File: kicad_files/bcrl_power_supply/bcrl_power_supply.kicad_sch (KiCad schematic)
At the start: 0 parts

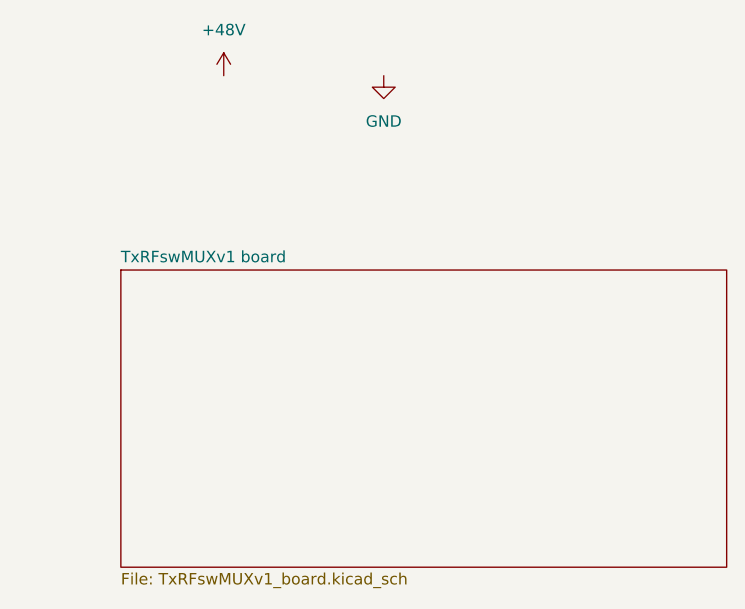
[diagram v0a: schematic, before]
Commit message: added decoupling
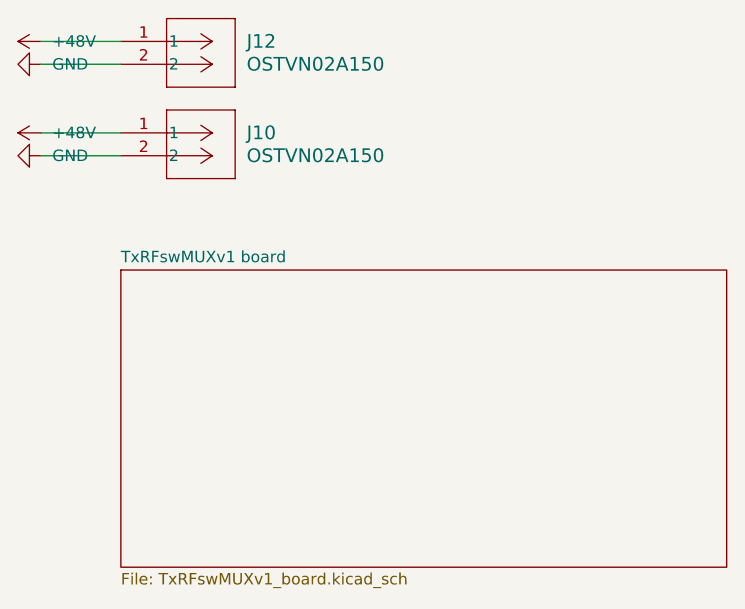
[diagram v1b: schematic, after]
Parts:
- added J10, J12: OSTVN02A150, symbol BCRL_power_supply:OSTVN02A150
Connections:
- net +48V: now also J10.1, J12.1
- net GND: now also J10.2, J12.2
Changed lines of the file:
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@@
 (kicad_sch (version 20230121) (generator eeschema)
   (paper "A4")
-  (symbol (lib_id "power:+48V") (at 50.8 27.94 0) (unit 1)
+  (wire (pts (xy 30.48 34.29) (xy 39.37 34.29))
+    (stroke (width 0) (type default))
+  )
+  (wire (pts (xy 30.48 24.13) (xy 39.37 24.13))
+    (stroke (width 0) (type default))
+  )
+  (wire (pts (xy 30.48 36.83) (xy 39.37 36.83))
+    (stroke (width 0) (type default))
+  )
+  (wire (pts (xy 30.48 26.67) (xy 39.37 26.67))
+    (stroke (width 0) (type default))
+  )
+  (symbol (lib_id "BCRL_power_supply:OSTVN02A150") (at 39.37 34.29 0) (unit 1)
     (in_bom yes) (on_board yes) (dnp no) (fields_autoplaced)
-    (property "Reference" "#PWR01" (at 50.8 31.75 0)
+    (property "Reference" "J10" (at 53.34 34.29 0)
+      (effects (font (size 1.524 1.524)) (justify left))
+    )
+    (property "Value" "OSTVN02A150" (at 53.34 36.83 0)
+      (effects (font (size 1.524 1.524)) (justify left))
+    )
+    (property "Footprint" "" (at 29.21 29.21 0)
+      (effects (font (size 1.27 1.27) italic) hide)
+    )
+    (property "Datasheet" "" (at 33.02 31.75 0)
+      (effects (font (size 1.27 1.27) italic) hide)
+    )
+    (pin "1")
+    (pin "2")
+    (instances
+      (project "bcrl_power_supply"
+        (path "/77f0f57c-9586-4625-9281-fa8cbd8015db"
+          (reference "J10") (unit 1)
+        )
+      )
+    )
+  )
+  (symbol (lib_id "power:+48V") (at 30.48 24.13 90) (unit 1)
+    (in_bom yes) (on_board yes) (dnp no) (fields_autoplaced)
+    (property "Reference" "#PWR090" (at 34.29 24.13 0)
       (effects (font (size 1.27 1.27)) hide)
     )
-    (property "Value" "+48V" (at 50.8 22.86 0)
-      (effects (font (size 1.27 1.27)))
+    (property "Value" "+48V" (at 31.75 24.13 90)
+      (effects (font (size 1.27 1.27)) (justify right))
     )
-    (property "Footprint" "" (at 50.8 27.94 0)
+    (property "Footprint" "" (at 30.48 24.13 0)
       (effects (font (size 1.27 1.27)) hide)
     )
-    (property "Datasheet" "" (at 50.8 27.94 0)
+    (property "Datasheet" "" (at 30.48 24.13 0)
+      (effects (font (size 1.27 1.27)) hide)
+    )
+    (pin "1")
+    (instances
+      (project "bcrl_power_supply"
+        (path "/77f0f57c-9586-4625-9281-fa8cbd8015db"
+          (reference "#PWR090") (unit 1)
+        )
+      )
+    )
+  )
+  (symbol (lib_id "power:+48V") (at 30.48 34.29 90) (unit 1)
+    (in_bom yes) (on_board yes) (dnp no) (fields_autoplaced)
+    (property "Reference" "#PWR01" (at 34.29 34.29 0)
+      (effects (font (size 1.27 1.27)) hide)
+    )
+    (property "Value" "+48V" (at 31.75 34.29 90)
+      (effects (font (size 1.27 1.27)) (justify right))
+    )
+    (property "Footprint" "" (at 30.48 34.29 0)
+      (effects (font (size 1.27 1.27)) hide)
+    )
+    (property "Datasheet" "" (at 30.48 34.29 0)
       (effects (font (size 1.27 1.27)) hide)
     )
@@
     )
   )
-  (symbol (lib_id "power:GND") (at 68.58 27.94 0) (unit 1)
+  (symbol (lib_id "power:GND") (at 30.48 26.67 270) (unit 1)
     (in_bom yes) (on_board yes) (dnp no) (fields_autoplaced)
-    (property "Reference" "#PWR02" (at 68.58 34.29 0)
+    (property "Reference" "#PWR091" (at 24.13 26.67 0)
       (effects (font (size 1.27 1.27)) hide)
     )
-    (property "Value" "GND" (at 68.58 33.02 0)
-      (effects (font (size 1.27 1.27)))
+    (property "Value" "GND" (at 31.75 26.67 90)
+      (effects (font (size 1.27 1.27)) (justify left))
     )
-    (property "Footprint" "" (at 68.58 27.94 0)
+    (property "Footprint" "" (at 30.48 26.67 0)
       (effects (font (size 1.27 1.27)) hide)
     )
-    (property "Datasheet" "" (at 68.58 27.94 0)
+    (property "Datasheet" "" (at 30.48 26.67 0)
+      (effects (font (size 1.27 1.27)) hide)
+    )
+    (pin "1")
+    (instances
+      (project "bcrl_power_supply"
+        (path "/77f0f57c-9586-4625-9281-fa8cbd8015db"
+          (reference "#PWR091") (unit 1)
+        )
+      )
+    )
+  )
+  (symbol (lib_id "power:GND") (at 30.48 36.83 270) (unit 1)
+    (in_bom yes) (on_board yes) (dnp no) (fields_autoplaced)
+    (property "Reference" "#PWR02" (at 24.13 36.83 0)
+      (effects (font (size 1.27 1.27)) hide)
+    )
+    (property "Value" "GND" (at 31.75 36.83 90)
+      (effects (font (size 1.27 1.27)) (justify left))
+    )
+    (property "Footprint" "" (at 30.48 36.83 0)
+      (effects (font (size 1.27 1.27)) hide)
+    )
+    (property "Datasheet" "" (at 30.48 36.83 0)
       (effects (font (size 1.27 1.27)) hide)
     )
@@
         )
       )
+    )
+  )
+  (symbol (lib_id "BCRL_power_supply:OSTVN02A150") (at 39.37 24.13 0) (unit 1)
+    (in_bom yes) (on_board yes) (dnp no) (fields_autoplaced)
+    (property "Reference" "J12" (at 53.34 24.13 0)
+      (effects (font (size 1.524 1.524)) (justify left))
+    )
+    (property "Value" "OSTVN02A150" (at 53.34 26.67 0)
+      (effects (font (size 1.524 1.524)) (justify left))
+    )
+    (property "Footprint" "" (at 29.21 19.05 0)
+      (effects (font (size 1.27 1.27) italic) hide)
+    )
+    (property "Datasheet" "" (at 33.02 21.59 0)
+      (effects (font (size 1.27 1.27) italic) hide)
+    )
+    (pin "1")
+    (pin "2")
+    (instances
+      (project "bcrl_power_supply"
+        (path "/77f0f57c-9586-4625-9281-fa8cbd8015db"
+          (reference "J12") (unit 1)
+        )
+      )
